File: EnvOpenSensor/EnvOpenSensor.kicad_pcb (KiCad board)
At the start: 2 copper layers, 89.7 x 67.5 mm, 64 parts, among them IC1 IS31FL3730-QFLS2-TR, IC2 IS31FL3730-QFLS2-TR, IC3 IS31FL3730-QFLS2-TR, IC4 IS31FL3730-QFLS2-TR, J1 HRO_TYPE-C-31-M-12, J2 AVR-ISP-6, SW1 SW_Push, SW2 SW_Push, SW3 SW_Push, SW4 SW_Push, U0 TCA9548ARGER, U1 SCD41-D-R2, U2 Si7021-A20, U3 LDO SOT-23-5 3.3V, U4 ATtiny85-20S

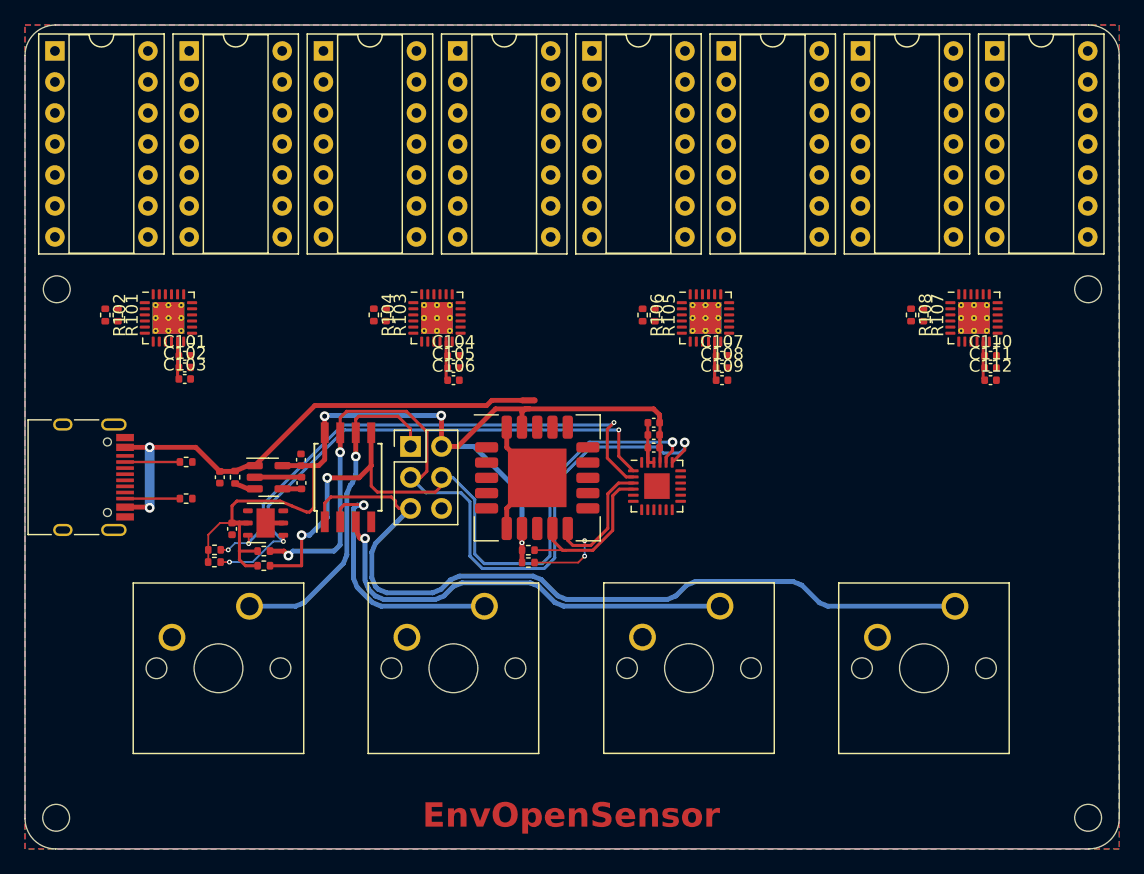
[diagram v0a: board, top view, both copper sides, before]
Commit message: re-did the PCB
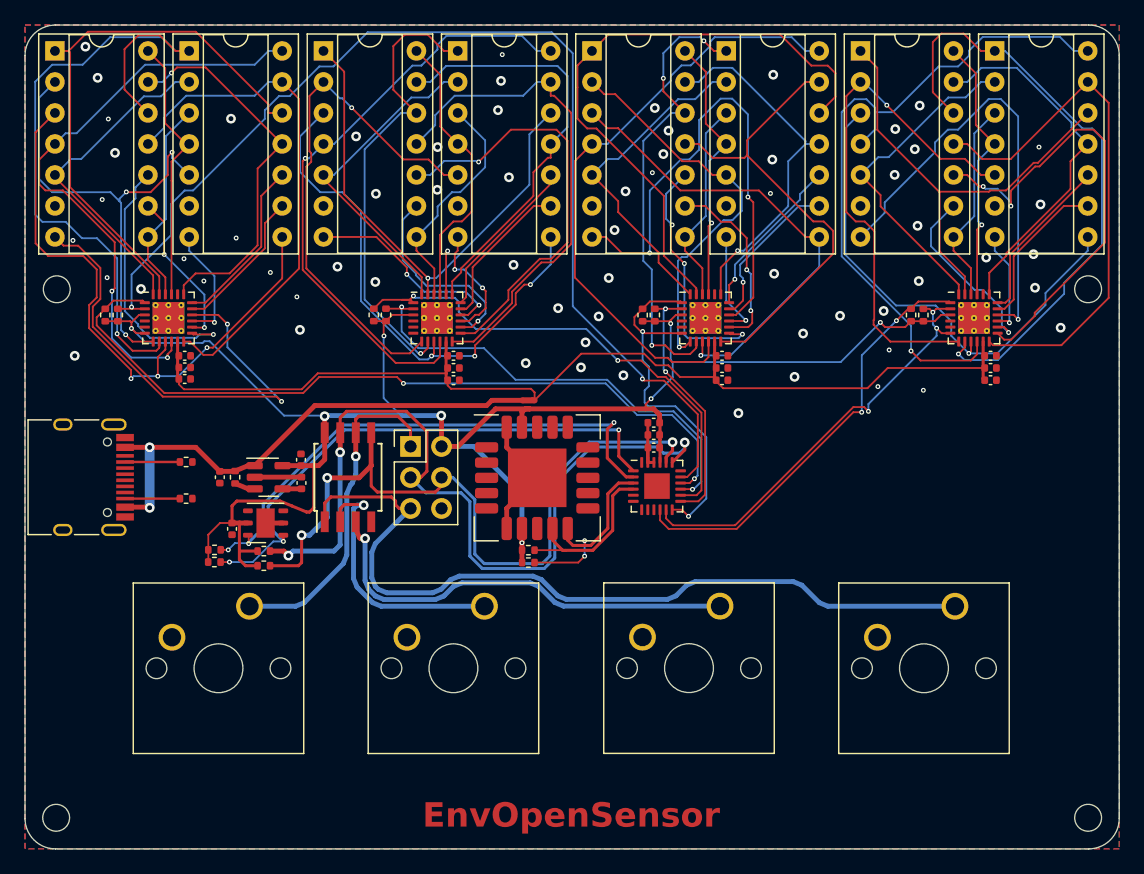
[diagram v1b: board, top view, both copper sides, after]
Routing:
- net SCL7_3V3: track 0.00 -> 92.8 mm, vias 0 -> 2
- net VCC: track 12.7 -> 85.6 mm
- net +3V3: track 84.8 -> 157.2 mm, vias 3 -> 8
- net SDA7_3V3: track 0.00 -> 64.0 mm, vias 0 -> 2
- net IC1R2: track 0.00 -> 56.9 mm, vias 0 -> 1
- net IC4R4: track 0.00 -> 56.5 mm, vias 0 -> 1
- net IC4R2: track 0.00 -> 50.6 mm, vias 0 -> 1
- net IC3C2: track 0.00 -> 50.5 mm
- net IC1R3: track 0.00 -> 50.1 mm, vias 0 -> 3
- net IC2R4: track 0.00 -> 50.1 mm, vias 0 -> 1
- net IC3R4: track 0.00 -> 49.9 mm
- net IC1R4: track 0.00 -> 48.4 mm, vias 0 -> 2
- net IC1C2: track 0.00 -> 45.5 mm
- net IC2R3: track 0.00 -> 44.6 mm, vias 0 -> 3
- net IC4R5: track 0.00 -> 44.0 mm
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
